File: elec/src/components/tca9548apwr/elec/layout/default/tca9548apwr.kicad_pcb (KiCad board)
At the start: 2 copper layers, 20 parts

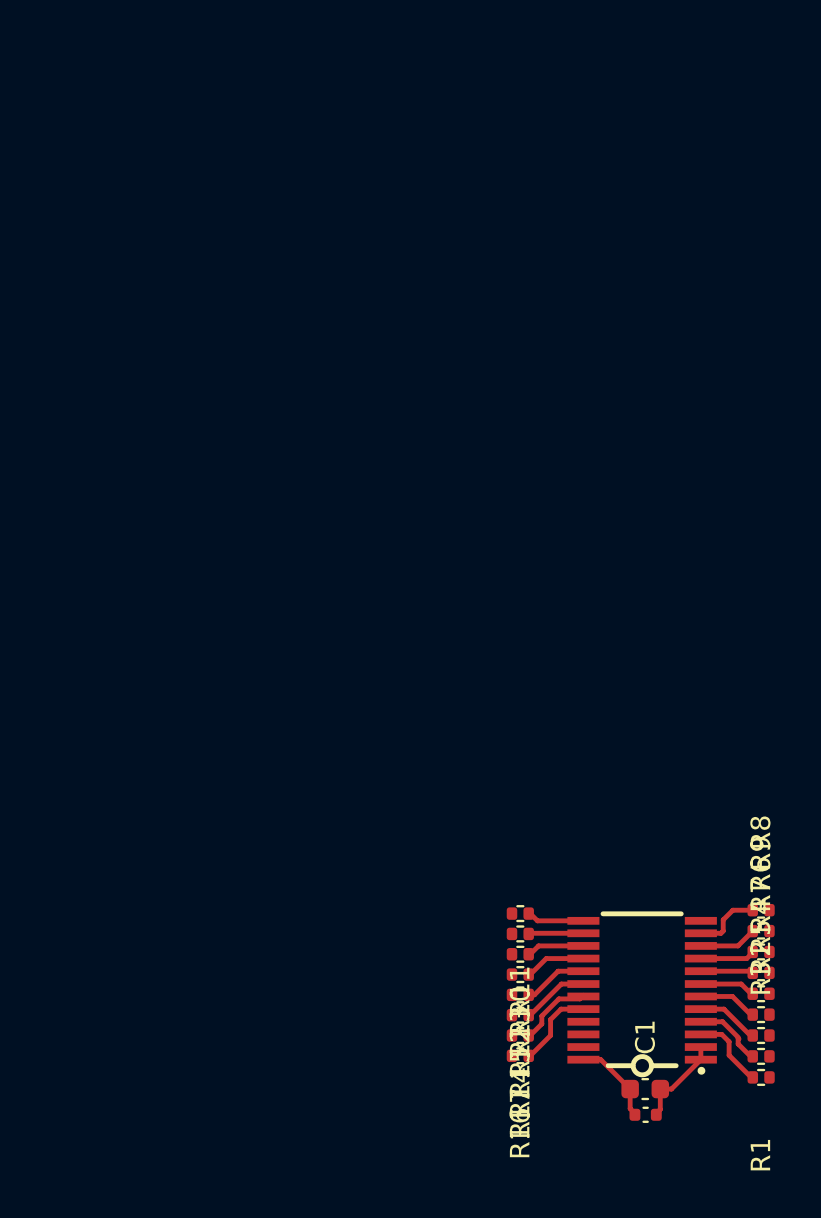
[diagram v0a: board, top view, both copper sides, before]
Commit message: replicate connection failure with two cells
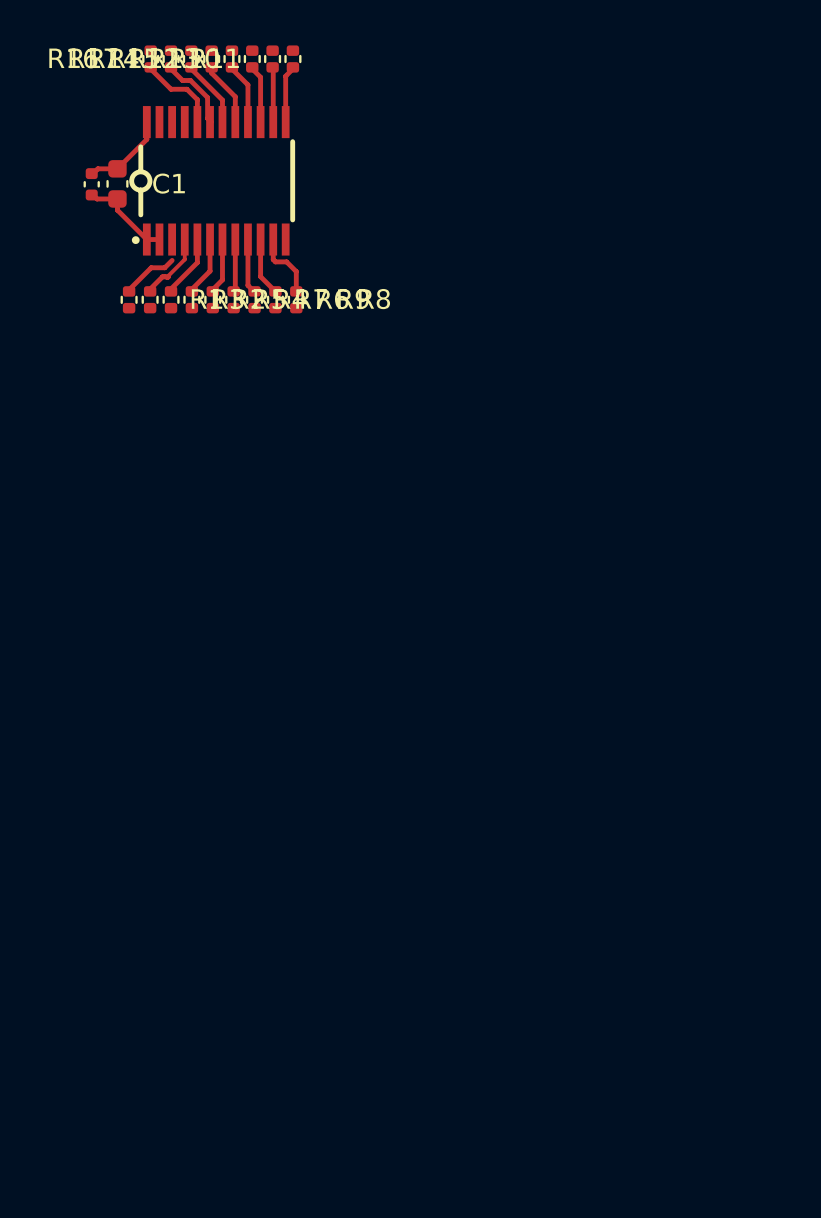
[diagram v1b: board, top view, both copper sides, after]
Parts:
- moved C1 55.7 mm to (100.0, 109.6), turned to -90 degrees
- moved R16 54.7 mm to (103.0, 103.1), turned to 90 degrees
- moved C2 53.9 mm to (101.3, 109.6), turned to -90 degrees
- moved R17 53.3 mm to (104.0, 103.1), turned to 90 degrees
- moved R14 52.0 mm to (105.1, 103.1), turned to 90 degrees
- moved R1 51.5 mm to (101.9, 115.5), turned to -90 degrees
- moved R15 50.7 mm to (106.1, 103.1), turned to 90 degrees
- moved R3 50.0 mm to (103.0, 115.5), turned to -90 degrees
- moved R12 49.4 mm to (107.2, 103.1), turned to 90 degrees
- moved R2 48.5 mm to (104.0, 115.5), turned to -90 degrees
- moved R13 48.1 mm to (108.2, 103.1), turned to 90 degrees
- moved U1 47.0 mm to (106.4, 109.4), turned to 0 degrees
- moved R5 47.0 mm to (105.1, 115.5), turned to -90 degrees
- moved R10 46.8 mm to (109.3, 103.1), turned to 90 degrees
- moved R4 45.5 mm to (106.2, 115.5), turned to -90 degrees
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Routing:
- net ic-scl-2: track 3.91 -> 0.00 mm
- net reset_: track 0.00 -> 2.84 mm
